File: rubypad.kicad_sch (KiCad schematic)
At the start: 33 parts, among them J1 HRO-TYPE-C, SW1 SW_Push, SW2 RotaryEncoder_Switch, U1 ATmega32U4-A, Y1 16MHz

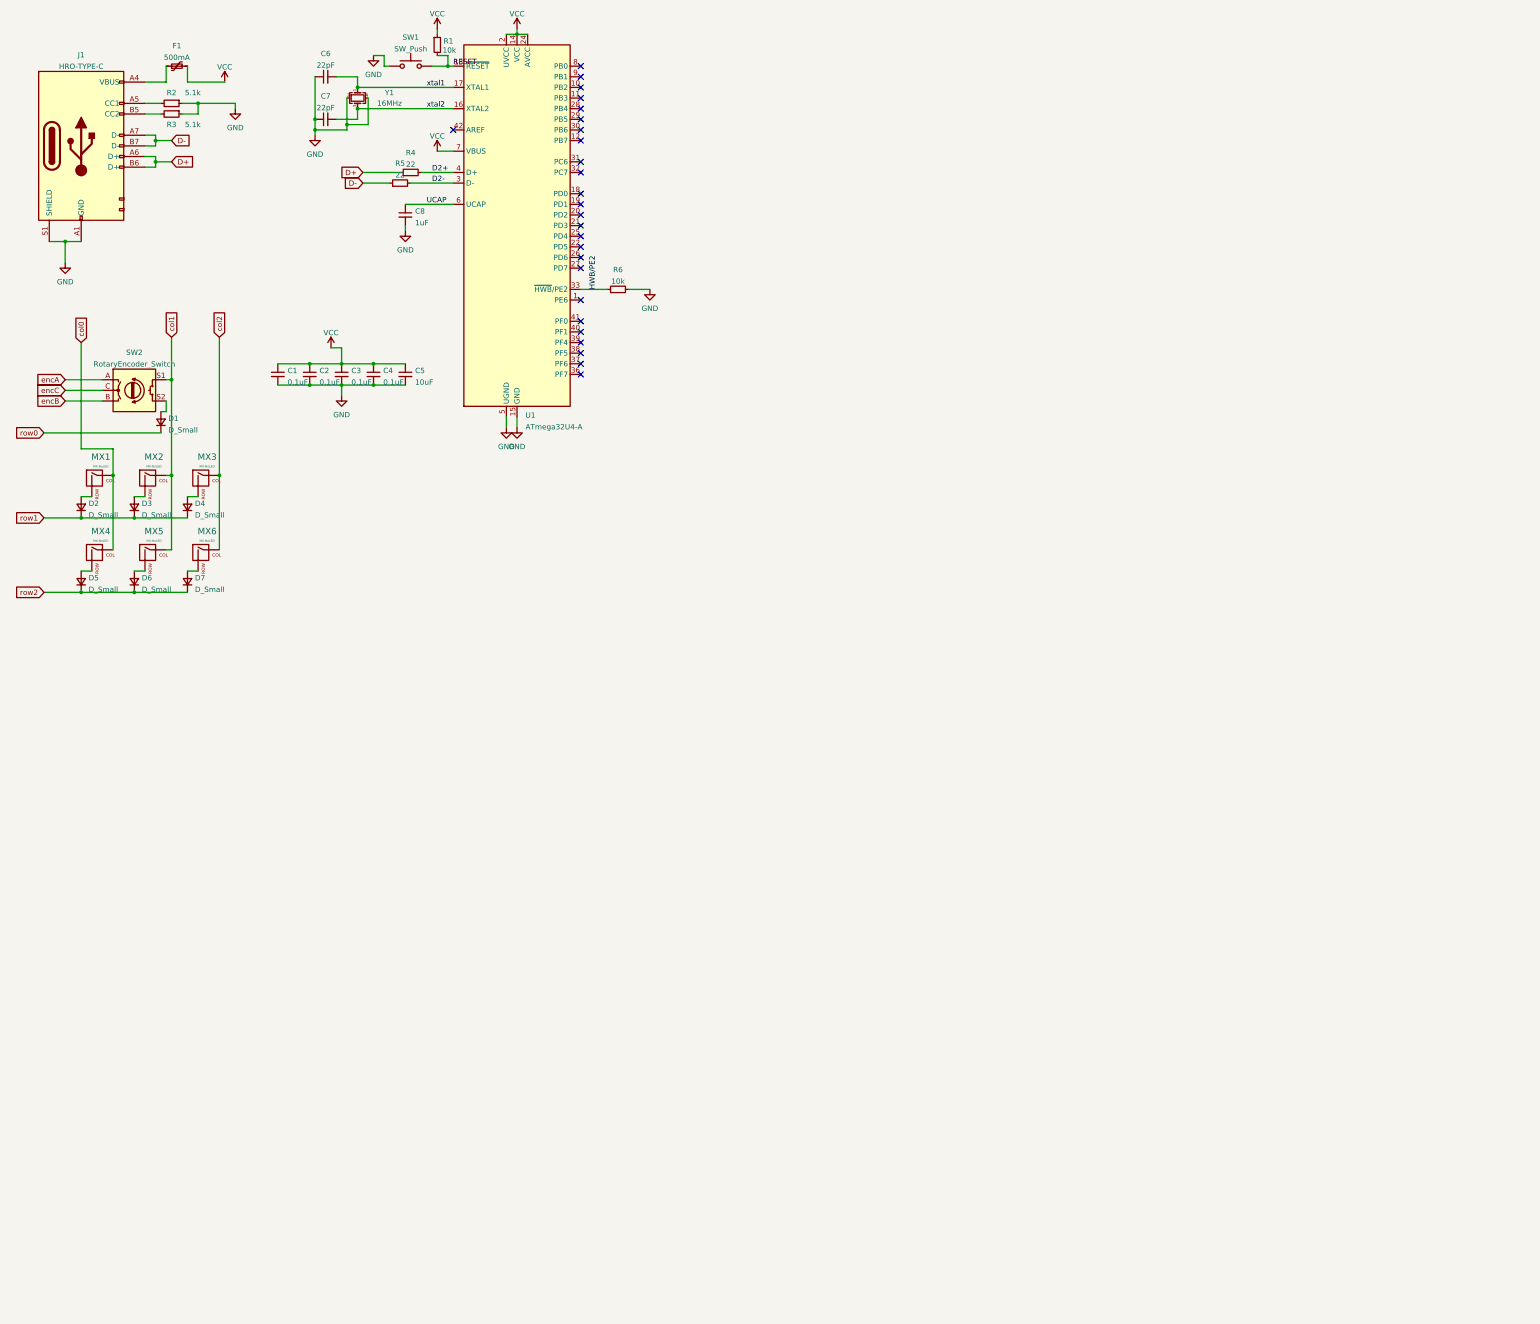
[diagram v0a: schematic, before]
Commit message: save changes
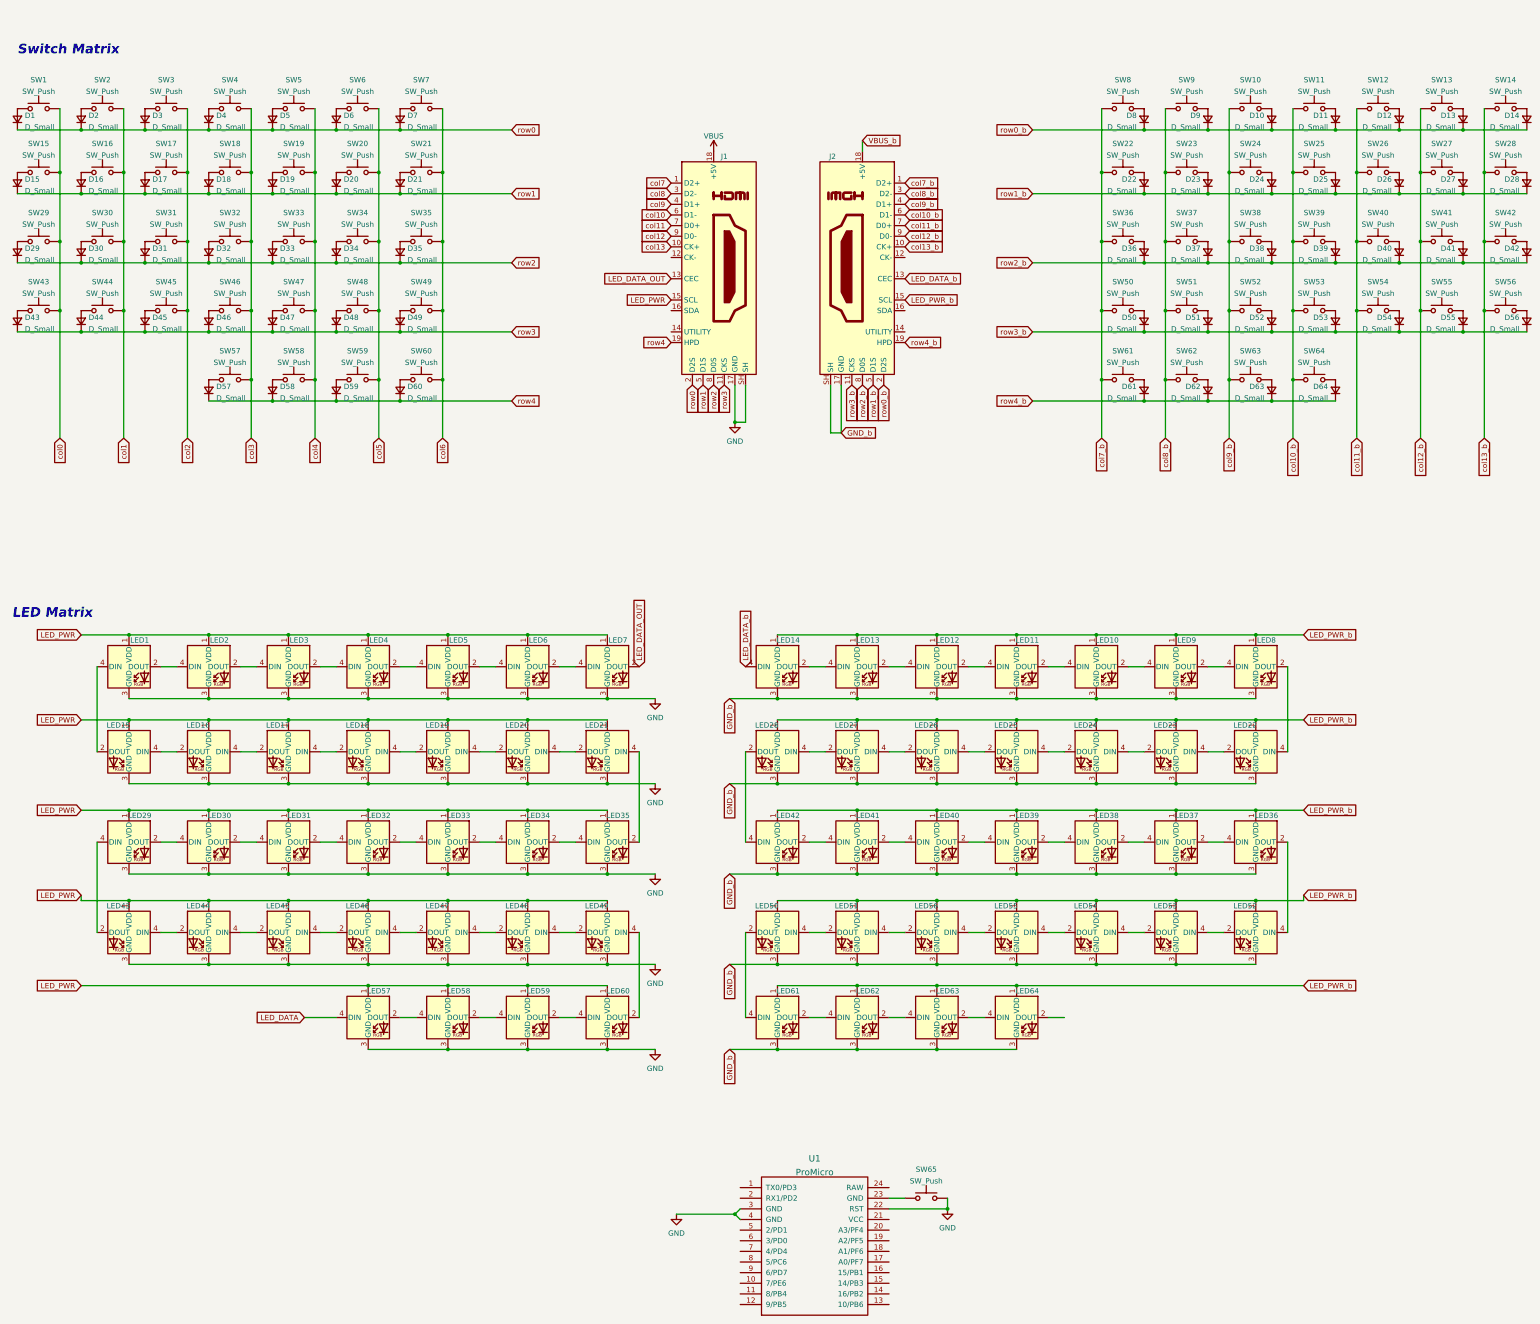
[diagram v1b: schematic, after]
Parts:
- removed C1, C2, C3, C4: 0.1uF, Capacitor_SMD:C_0805_2012Metric_Pad1.18x1.45mm_HandSolder, symbol Device:C_Small
- removed C5: 10uF, Capacitor_SMD:C_0805_2012Metric_Pad1.18x1.45mm_HandSolder, symbol Device:C_Small
- removed C6, C7: 22pF, Capacitor_SMD:C_0805_2012Metric_Pad1.18x1.45mm_HandSolder, symbol Device:C_Small
- removed C8: 1uF, Capacitor_SMD:C_0805_2012Metric_Pad1.18x1.45mm_HandSolder, symbol Device:C_Small
- removed F1: 500mA, Fuse:Fuse_1206_3216Metric_Pad1.42x1.75mm_HandSolder, symbol Device:Polyfuse_Small
- removed J1: HRO-TYPE-C, reversible-kicad-footprints:HRO-TYPE-C-31-M-12-HandSoldering-NoSBU, symbol reversible-kicad-symbols:HRO-TYPE-C-31-M-12-HandSoldering-NoSBU
- removed MX1, MX2, MX3, MX4, MX5, MX6: MX-NoLED, MX_Only:MXOnly-1U-Hotswap, symbol MX_Alps_Hybrid:MX-NoLED
- removed R1, R6: 10k, Resistor_SMD:R_0805_2012Metric_Pad1.20x1.40mm_HandSolder, symbol Device:R_Small
- removed R2, R3: 5.1k, Resistor_SMD:R_0805_2012Metric_Pad1.20x1.40mm_HandSolder, symbol Device:R_Small
- removed R4, R5: 22, Resistor_SMD:R_0805_2012Metric_Pad1.20x1.40mm_HandSolder, symbol Device:R_Small
- removed SW2: RotaryEncoder_Switch, reversible-kicad-footprints:EC11_Switch, symbol Device:RotaryEncoder_Switch
- removed U1: ATmega32U4-A, Package_QFP:TQFP-44_10x10mm_P0.8mm, symbol MCU_Microchip_ATmega:ATmega32U4-A
- removed Y1: 16MHz, Crystal:Crystal_SMD_SeikoEpson_TSX3225-4Pin_3.2x2.5mm_HandSoldering, symbol Device:Crystal_GND24_Small
- added D10, D11, D12, D13, D14, D15, D16, D17, D18, D19, D20, D21, D22, D23, D24, D25, D26, D27, D28, D29, D30, D31, D32, D33, D34, D35, D36, D37, D38, D39, D40, D41, D42, D43, D44, D45, D46, D47, D48, D49, D50, D51, D52, D53, D54, D55, D56, D57, D58, D59, D60, D61, D62, D63, D64, D8, D9: D_Small, reversible-kicad-footprints:D_SOD-123, symbol Device:D_Small
- added J1, J2: HDMI_A, Connector_HDMI:HDMI_A_Contact_Technology_HDMI-19APL2_Horizontal, symbol Connector:HDMI_A
- added LED1, LED10, LED11, LED12, LED13, LED14, LED15, LED16, LED17, LED18, LED19, LED2, LED20, LED21, LED22, LED23, LED24, LED25, LED26, LED27, LED28, LED29, LED3, LED30, LED31, LED32, LED33, LED34, LED35, LED36, LED37, LED38, LED39, LED4, LED40, LED41, LED42, LED43, LED44, LED45, LED46, LED47, LED48, LED49, LED5, LED50, LED51, LED52, LED53, LED54, LED55, LED56, LED57, LED58, LED59, LED6, LED60, LED61, LED62, LED63, LED64, LED7, LED8, LED9: SK6812Mini-E, reversible-kicad-footprints:SK6812Mini-E, symbol DjinnSymbols:SK6812Mini-E
- added SW10, SW11, SW12, SW13, SW14, SW15, SW16, SW17, SW18, SW19, SW2, SW20, SW21, SW22, SW23, SW24, SW25, SW26, SW27, SW28, SW29, SW3, SW30, SW31, SW32, SW33, SW34, SW35, SW36, SW37, SW38, SW39, SW4, SW40, SW41, SW42, SW43, SW44, SW45, SW46, SW47, SW48, SW49, SW5, SW50, SW51, SW52, SW53, SW54, SW55, SW56, SW57, SW58, SW59, SW6, SW60, SW61, SW62, SW63, SW64, SW7, SW8, SW9: SW_Push, reversible-kicad-footprints:MX-1U-Hotswap, symbol Switch:SW_Push
- added SW65: SW_Push, reversible-kicad-footprints:PushButton_4.5mm, symbol Switch:SW_Push
- added U1: ProMicro, Keebio-Parts:ArduinoProMicro, symbol keebio:ProMicro
- SW1: footprint reversible-kicad-footprints:PushButton_4.5mm -> reversible-kicad-footprints:MX-1U-Hotswap
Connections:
- net RESET is gone; now on net col0: SW1.2
- net GND: now also J1.17 (GND), J1.SH, LED1.3 (GND), LED15.3 (GND), LED16.3 (GND), LED17.3 (GND), LED18.3 (GND), LED19.3 (GND), LED2.3 (GND), LED20.3 (GND), LED21.3 (GND), LED29.3 (GND), LED3.3 (GND), LED30.3 (GND), LED31.3 (GND), LED32.3 (GND), LED33.3 (GND), LED34.3 (GND), LED35.3 (GND), LED4.3 (GND), LED43.3 (GND), LED44.3 (GND), LED45.3 (GND), LED46.3 (GND), LED47.3 (GND), LED48.3 (GND), LED49.3 (GND), LED5.3 (GND), LED57.3 (GND), LED58.3 (GND), LED59.3 (GND), LED6.3 (GND), LED60.3 (GND), LED7.3 (GND), SW65.2, U1.22 (RST), U1.3 (GND), U1.4 (GND); no longer SW1.1
- net col0: now also SW15.2, SW29.2, SW43.2
- net col1: now also SW16.2, SW2.2, SW30.2, SW44.2
- net col2: now also SW17.2, SW3.2, SW31.2, SW45.2
- net row0: now also D2.1 (K), D3.1 (K), D4.1 (K), D5.1 (K), D6.1 (K), D7.1 (K), J1.2 (D2S)
- net row1: now also D15.1 (K), D16.1 (K), D17.1 (K), D18.1 (K), D19.1 (K), D20.1 (K), D21.1 (K), J1.5 (D1S); no longer D2.1 (K), D3.1 (K), D4.1 (K)
- net row2: now also D29.1 (K), D30.1 (K), D31.1 (K), D32.1 (K), D33.1 (K), D34.1 (K), D35.1 (K), J1.8 (D0S); no longer D5.1 (K), D6.1 (K), D7.1 (K)
- net at D2.2 (A): now also SW2.1
- net at D3.2 (A): now also SW3.1
- net at D6.2 (A): now also SW6.1
- net at D4.2 (A): now also SW4.1
- net at D5.2 (A): now also SW5.1
- net at D1.2 (A): now also SW1.1
- net at D7.2 (A): now also SW7.1
- new net: D22.2 (A), SW22.1
- new net: LED21.4 (DIN), LED35.2 (DOUT)
- new net: LED34.2 (DOUT), LED35.4 (DIN)
- new net: D10.2 (A), SW10.1
- new net: LED19.4 (DIN), LED20.2 (DOUT)
- new net: LED20.4 (DIN), LED21.2 (DOUT)
- new net: D62.2 (A), SW62.1
- new net: D41.2 (A), SW41.1
- new net: LED16.4 (DIN), LED17.2 (DOUT)
- new net: LED17.4 (DIN), LED18.2 (DOUT)
- new net: D8.2 (A), SW8.1
- new net: D23.2 (A), SW23.1
- new net: LED62.2 (DOUT), LED63.4 (DIN)
- new net: LED61.2 (DOUT), LED62.4 (DIN)
- new net: D26.2 (A), SW26.1
- new net: D21.2 (A), SW21.1
- new net: LED31.2 (DOUT), LED32.4 (DIN)
- new net: LED30.2 (DOUT), LED31.4 (DIN)
- new net: D56.2 (A), SW56.1
- new net: LED33.2 (DOUT), LED34.4 (DIN)
- new net: D27.2 (A), SW27.1
- new net: D14.2 (A), SW14.1
- new net: D15.2 (A), SW15.1
- new net: LED36.4 (DIN), LED37.2 (DOUT)
- new net: LED37.4 (DIN), LED38.2 (DOUT)
- new net: LED45.4 (DIN), LED46.2 (DOUT)
- new net: LED46.4 (DIN), LED47.2 (DOUT)
- new net: LED51.4 (DIN), LED56.2 (DOUT)
- new net: LED55.2 (DOUT), LED56.4 (DIN)
- new net: LED25.2 (DOUT), LED26.4 (DIN)
- new net: LED24.2 (DOUT), LED25.4 (DIN)
- new net: D64.2 (A), SW64.1
- new net: LED18.4 (DIN), LED19.2 (DOUT)
- new net: SW65.1, U1.23 (GND)
- new net: D52.2 (A), SW52.1
- new net: LED12.4 (DIN), LED13.2 (DOUT)
- new net: LED13.4 (DIN), LED14.2 (DOUT)
- new net: D45.2 (A), SW45.1
- new net: LED54.2 (DOUT), LED55.4 (DIN)
- new net: LED53.2 (DOUT), LED54.4 (DIN)
- new net: D40.2 (A), SW40.1
- new net: D34.2 (A), SW34.1
- new net: D54.2 (A), SW54.1
- new net: D53.2 (A), SW53.1
- new net: LED58.2 (DOUT), LED59.4 (DIN)
- new net: LED57.2 (DOUT), LED58.4 (DIN)
- new net: LED11.4 (DIN), LED12.2 (DOUT)
- new net: D43.2 (A), SW43.1
- new net: D44.2 (A), SW44.1
- new net: D42.2 (A), SW42.1
- new net: LED1.4 (DIN), LED15.2 (DOUT)
- new net: LED15.4 (DIN), LED16.2 (DOUT)
- new net: D12.2 (A), SW12.1
- new net: D61.2 (A), SW61.1
- new net: LED38.4 (DIN), LED39.2 (DOUT)
- new net: D31.2 (A), SW31.1
- new net: D57.2 (A), SW57.1
- new net: D29.2 (A), SW29.1
- new net: LED29.2 (DOUT), LED30.4 (DIN)
- new net: LED29.4 (DIN), LED43.2 (DOUT)
- new net: D33.2 (A), SW33.1
- new net: D46.2 (A), SW46.1
- new net: D39.2 (A), SW39.1
- new net: D50.2 (A), SW50.1
- new net: D35.2 (A), SW35.1
- new net: D19.2 (A), SW19.1
- new net: LED32.2 (DOUT), LED33.4 (DIN)
- new net: D47.2 (A), SW47.1
- new net: D13.2 (A), SW13.1
- new net: LED3.2 (DOUT), LED4.4 (DIN)
- new net: LED2.2 (DOUT), LED3.4 (DIN)
- new net: D38.2 (A), SW38.1
- new net: D63.2 (A), SW63.1
- new net: LED43.4 (DIN), LED44.2 (DOUT)
- new net: D11.2 (A), SW11.1
- new net: D51.2 (A), SW51.1
- new net: LED28.2 (DOUT), LED42.4 (DIN)
- new net: LED27.2 (DOUT), LED28.4 (DIN)
- new net: D24.2 (A), SW24.1
- new net: D9.2 (A), SW9.1
- new net: LED1.2 (DOUT), LED2.4 (DIN)
- new net: D17.2 (A), SW17.1
- new net: LED63.2 (DOUT), LED64.4 (DIN)
- new net: LED10.4 (DIN), LED11.2 (DOUT)
- new net: LED36.2 (DOUT), LED52.4 (DIN)
- new net: D55.2 (A), SW55.1
- new net: D49.2 (A), SW49.1
- new net: D59.2 (A), SW59.1
- new net: LED50.2 (DOUT), LED61.4 (DIN)
- new net: LED50.4 (DIN), LED51.2 (DOUT)
- new net: D18.2 (A), SW18.1
- new net: D58.2 (A), SW58.1
- new net: LED49.4 (DIN), LED60.2 (DOUT)
- new net: LED59.2 (DOUT), LED60.4 (DIN)
- new net: D30.2 (A), SW30.1
- new net: LED26.2 (DOUT), LED27.4 (DIN)
- new net: LED39.4 (DIN), LED40.2 (DOUT)
- new net: D36.2 (A), SW36.1
- new net: D20.2 (A), SW20.1
- new net: LED8.4 (DIN), LED9.2 (DOUT)
- new net: LED10.2 (DOUT), LED9.4 (DIN)
- new net: LED47.4 (DIN), LED48.2 (DOUT)
- new net: LED48.4 (DIN), LED49.2 (DOUT)
- new net: LED40.4 (DIN), LED41.2 (DOUT)
- new net: LED41.4 (DIN), LED42.2 (DOUT)
- new net: D28.2 (A), SW28.1
- new net: D60.2 (A), SW60.1
- new net: D37.2 (A), SW37.1
- new net: D16.2 (A), SW16.1
- new net: D48.2 (A), SW48.1
- new net: D25.2 (A), SW25.1
- new net: LED23.2 (DOUT), LED24.4 (DIN)
- new net: LED22.2 (DOUT), LED23.4 (DIN)
- new net: LED5.2 (DOUT), LED6.4 (DIN)
- new net: LED4.2 (DOUT), LED5.4 (DIN)
- new net: LED52.2 (DOUT), LED53.4 (DIN)
- new net: LED22.4 (DIN), LED8.2 (DOUT)
- new net: LED44.4 (DIN), LED45.2 (DOUT)
- new net: D32.2 (A), SW32.1
- new net: LED6.2 (DOUT), LED7.4 (DIN)
- new net GND_b: J2.17 (GND), J2.SH, LED10.3 (GND), LED11.3 (GND), LED12.3 (GND), LED13.3 (GND), LED14.3 (GND), LED22.3 (GND), LED23.3 (GND), LED24.3 (GND), LED25.3 (GND), LED26.3 (GND), LED27.3 (GND), LED28.3 (GND), LED36.3 (GND), LED37.3 (GND), LED38.3 (GND), LED39.3 (GND), LED40.3 (GND), LED41.3 (GND), LED42.3 (GND), LED50.3 (GND), LED51.3 (GND), LED52.3 (GND), LED53.3 (GND), LED54.3 (GND), LED55.3 (GND), LED56.3 (GND), LED61.3 (GND), LED62.3 (GND), LED63.3 (GND), LED64.3 (GND), LED8.3 (GND), LED9.3 (GND)
- new net LED_DATA: LED57.4 (DIN)
- new net LED_DATA_OUT: J1.13 (CEC), LED7.2 (DOUT)
- new net LED_DATA_b: J2.13 (CEC), LED14.4 (DIN)
- new net LED_PWR: J1.15 (SCL), LED1.1 (VDD), LED15.1 (VDD), LED16.1 (VDD), LED17.1 (VDD), LED18.1 (VDD), LED19.1 (VDD), LED2.1 (VDD), LED20.1 (VDD), LED21.1 (VDD), LED29.1 (VDD), LED3.1 (VDD), LED30.1 (VDD), LED31.1 (VDD), LED32.1 (VDD), LED33.1 (VDD), LED34.1 (VDD), LED35.1 (VDD), LED4.1 (VDD), LED43.1 (VDD), LED44.1 (VDD), LED45.1 (VDD), LED46.1 (VDD), LED47.1 (VDD), LED48.1 (VDD), LED49.1 (VDD), LED5.1 (VDD), LED57.1 (VDD), LED58.1 (VDD), LED59.1 (VDD), LED6.1 (VDD), LED60.1 (VDD), LED7.1 (VDD)
- new net LED_PWR_b: J2.15 (SCL), LED10.1 (VDD), LED11.1 (VDD), LED12.1 (VDD), LED13.1 (VDD), LED14.1 (VDD), LED22.1 (VDD), LED23.1 (VDD), LED24.1 (VDD), LED25.1 (VDD), LED26.1 (VDD), LED27.1 (VDD), LED28.1 (VDD), LED36.1 (VDD), LED37.1 (VDD), LED38.1 (VDD), LED39.1 (VDD), LED40.1 (VDD), LED41.1 (VDD), LED42.1 (VDD), LED50.1 (VDD), LED51.1 (VDD), LED52.1 (VDD), LED53.1 (VDD), LED54.1 (VDD), LED55.1 (VDD), LED56.1 (VDD), LED61.1 (VDD), LED62.1 (VDD), LED63.1 (VDD), LED64.1 (VDD), LED8.1 (VDD), LED9.1 (VDD)
- new net VBUS: J1.18 (+5V)
- new net VBUS_b: J2.18 (+5V)
- new net col10: J1.6 (D1-)
- new net col10_b: J2.6 (D1-), SW11.2, SW25.2, SW39.2, SW53.2, SW64.2
- new net col11: J1.7 (D0+)
- new net col11_b: J2.7 (D0+), SW12.2, SW26.2, SW40.2, SW54.2
- new net col12: J1.9 (D0-)
- new net col12_b: J2.9 (D0-), SW13.2, SW27.2, SW41.2, SW55.2
- new net col13: J1.10 (CK+)
- new net col13_b: J2.10 (CK+), SW14.2, SW28.2, SW42.2, SW56.2
- new net col3: SW18.2, SW32.2, SW4.2, SW46.2, SW57.2
- new net col4: SW19.2, SW33.2, SW47.2, SW5.2, SW58.2
- new net col5: SW20.2, SW34.2, SW48.2, SW59.2, SW6.2
- new net col6: SW21.2, SW35.2, SW49.2, SW60.2, SW7.2
- new net col7: J1.1 (D2+)
- new net col7_b: J2.1 (D2+), SW22.2, SW36.2, SW50.2, SW61.2, SW8.2
- new net col8: J1.3 (D2-)
- new net col8_b: J2.3 (D2-), SW23.2, SW37.2, SW51.2, SW62.2, SW9.2
- new net col9: J1.4 (D1+)
- new net col9_b: J2.4 (D1+), SW10.2, SW24.2, SW38.2, SW52.2, SW63.2
- new net row0_b: D10.1 (K), D11.1 (K), D12.1 (K), D13.1 (K), D14.1 (K), D8.1 (K), D9.1 (K), J2.2 (D2S)
- new net row1_b: D22.1 (K), D23.1 (K), D24.1 (K), D25.1 (K), D26.1 (K), D27.1 (K), D28.1 (K), J2.5 (D1S)
- new net row2_b: D36.1 (K), D37.1 (K), D38.1 (K), D39.1 (K), D40.1 (K), D41.1 (K), D42.1 (K), J2.8 (D0S)
- new net row3: D43.1 (K), D44.1 (K), D45.1 (K), D46.1 (K), D47.1 (K), D48.1 (K), D49.1 (K), J1.11 (CKS)
- new net row3_b: D50.1 (K), D51.1 (K), D52.1 (K), D53.1 (K), D54.1 (K), D55.1 (K), D56.1 (K), J2.11 (CKS)
- new net row4: D57.1 (K), D58.1 (K), D59.1 (K), D60.1 (K), J1.19 (HPD)
- new net row4_b: D61.1 (K), D62.1 (K), D63.1 (K), D64.1 (K), J2.19 (HPD)
- no-connect marks 26 -> 0
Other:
- note added: "LED Matrix"
- note added: "Switch Matrix"
